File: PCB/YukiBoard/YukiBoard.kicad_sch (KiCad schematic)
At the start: 61 parts, among them J1 Conn_01x02, J2 Conn_01x02, SW1 SW_Push_45deg, SW10 SW_Push_45deg, SW11 SW_Push_45deg, SW12 SW_Push_45deg, SW13 SW_Push_45deg, SW14 SW_Push_45deg, SW15 SW_Push_45deg, SW16 SW_Push_45deg, SW17 SW_Push_45deg, SW18 SW_Push_45deg, SW19 SW_Push_45deg, SW2 SW_Push_45deg, SW20 SW_Push_45deg, SW21 SW_Push_45deg, SW22 SW_Push_45deg, SW23 SW_Push_45deg, SW24 SW_Push_45deg, SW25 SW_Push_45deg, SW26 SW_Push_45deg, SW27 SW_Push_45deg, SW28 SW_Push_45deg, SW29 SW_Push_45deg, SW3 SW_Push_45deg, SW30 SW_Push_45deg, SW31 SW_Push_45deg, SW32 SW_Push_45deg, SW33 SW_Push_45deg, SW34 SW_Push_45deg, SW35 SW_Push_45deg, SW36 SW_Push_45deg, SW37 SW_Push_45deg, SW38 SW_Push_45deg, SW39 SW_SPDT, SW4 SW_Push_45deg, SW5 SW_Push_45deg, SW6 SW_Push_45deg, SW7 SW_Push_45deg, SW8 SW_Push_45deg, SW9 SW_Push_45deg, U1 XIAO-nRF52840-DIP

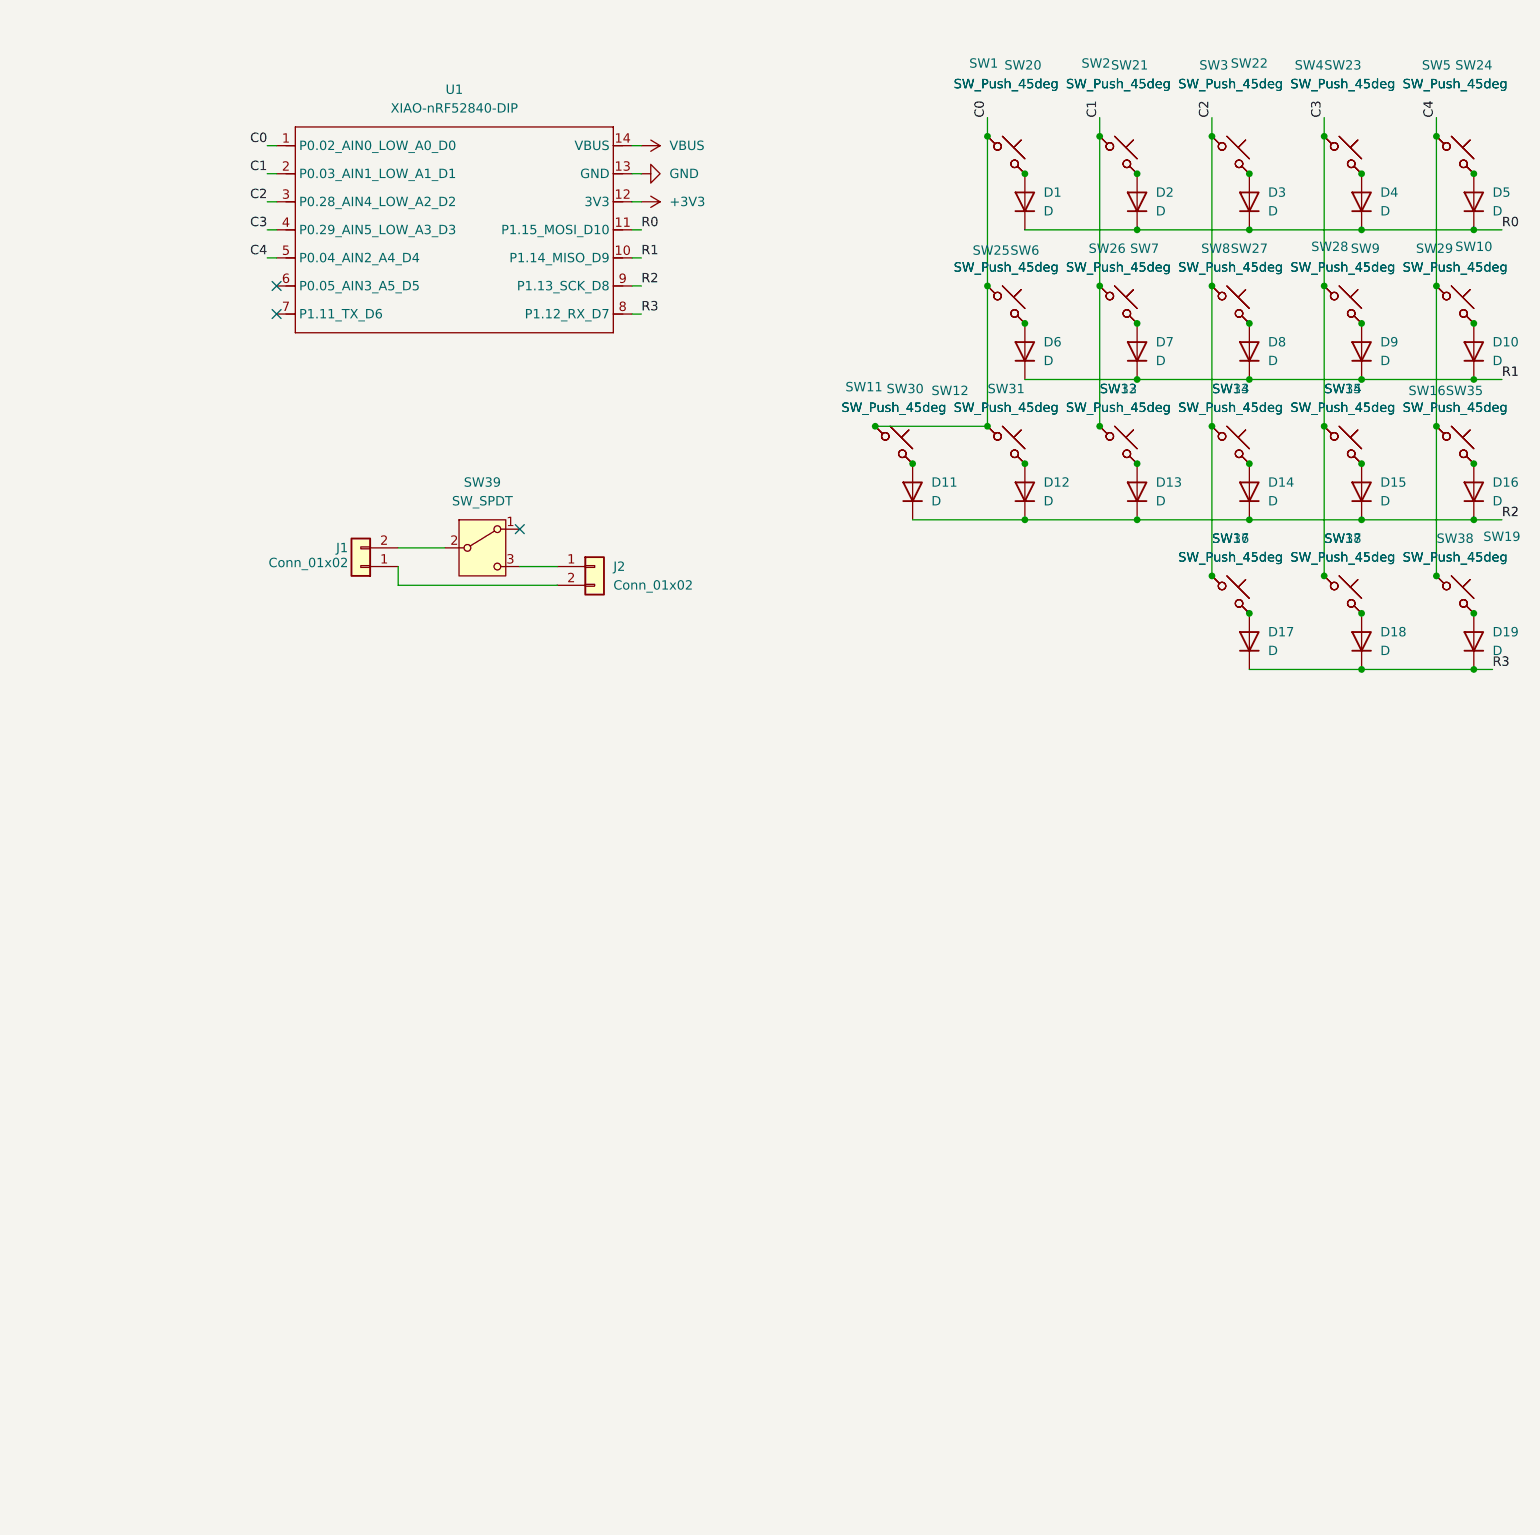
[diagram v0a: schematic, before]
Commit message: Add cool stuff to pcb 󰇳
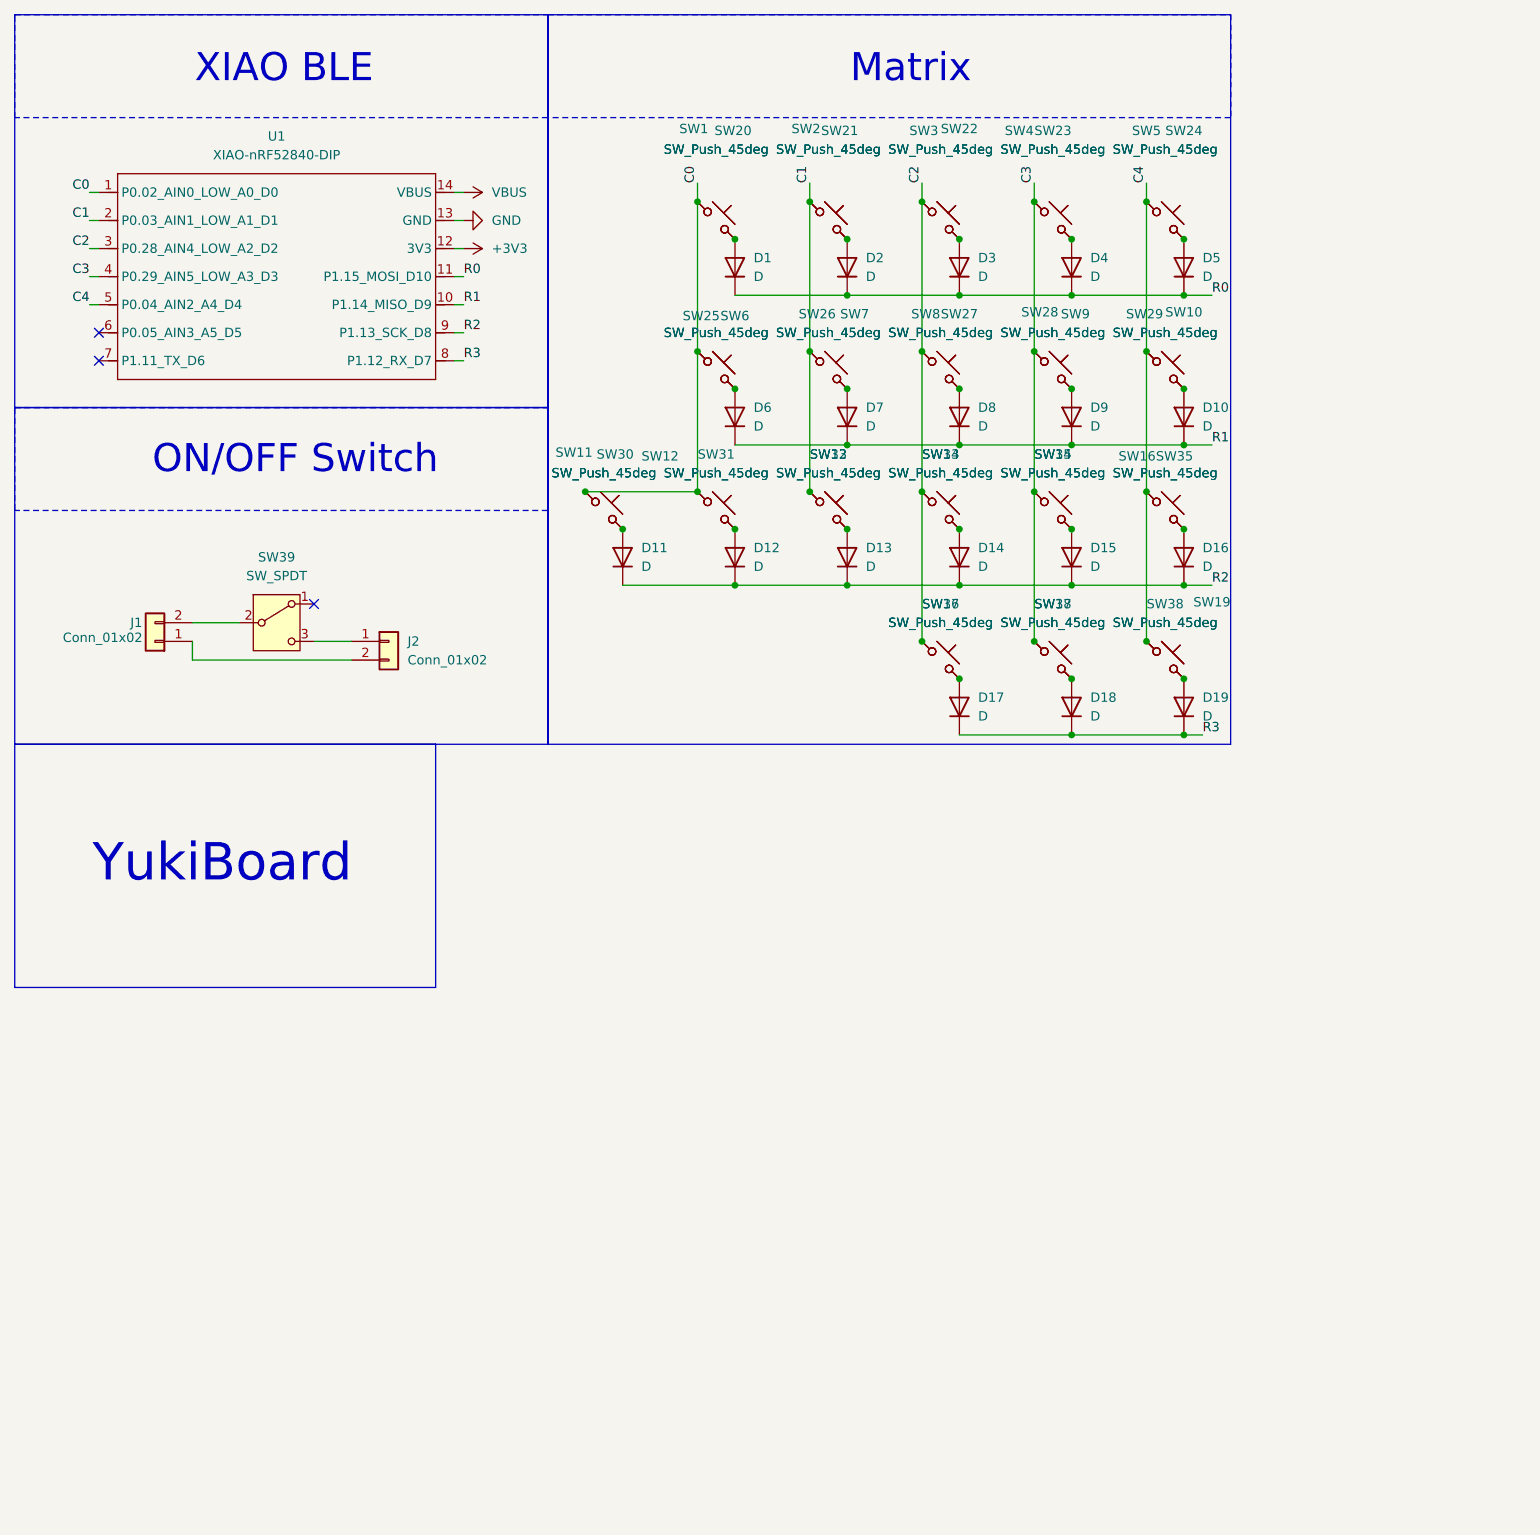
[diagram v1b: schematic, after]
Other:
- note added: "Matrix"
- note added: "ON/OFF Switch"
- note added: "XIAO BLE"
- note added: "YukiBoard"
- company: (none) -> manni
- title: (none) -> YukiBoard
- moved on the sheet: D1, D10, D11, D12, D13, D14, D15, D16, D17, D18, D19, D2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

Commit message: Add stuf
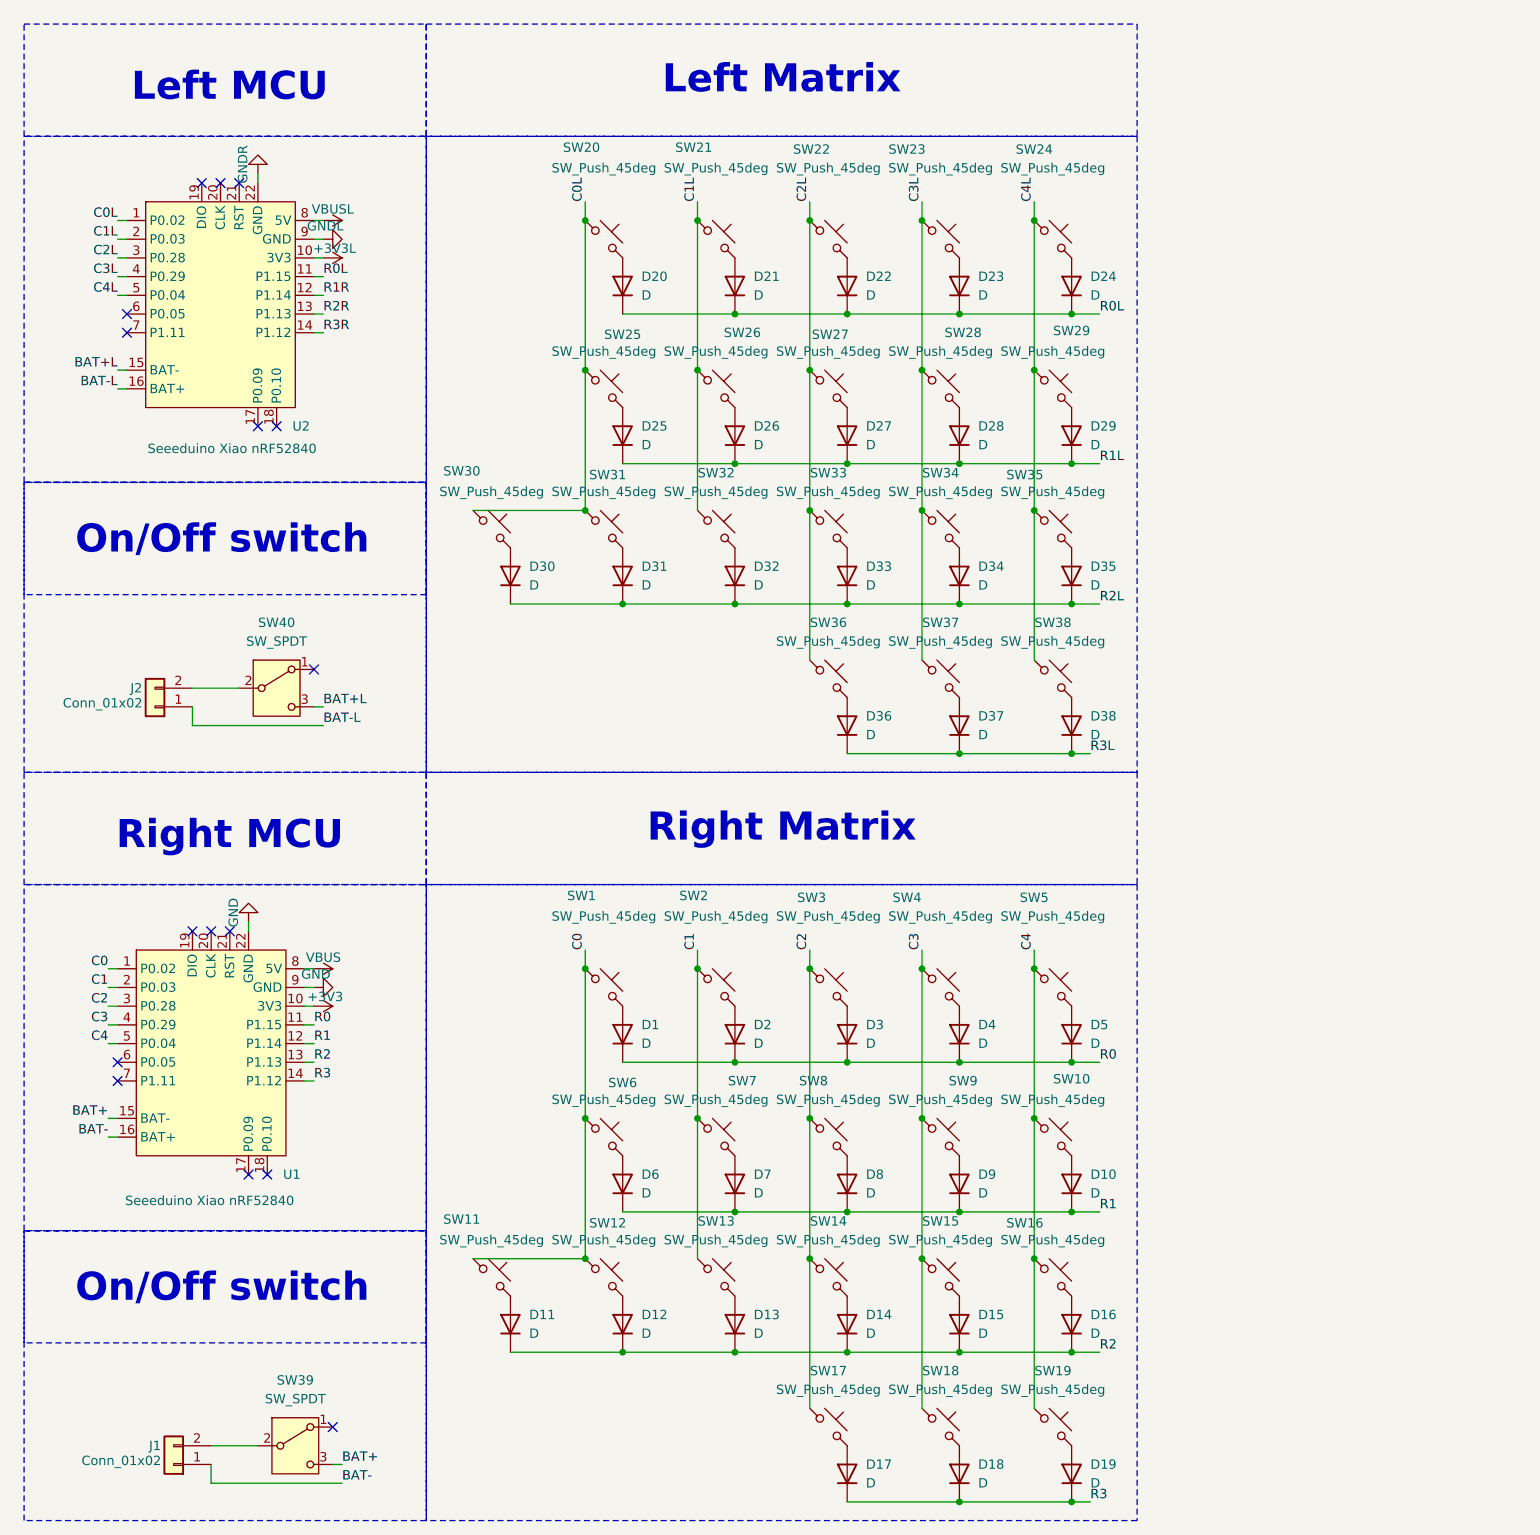
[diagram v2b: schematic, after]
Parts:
- removed U1: XIAO-nRF52840-DIP, XIAO-:XIAO-nRF52840-DIP, symbol Seeed_Studio_XIAO_Series:XIAO-nRF52840-DIP
- added D20, D21, D22, D23, D24, D25, D26, D27, D28, D29, D30, D31, D32, D33, D34, D35, D36, D37, D38: D, Diode_SMD:D_SOD-123, symbol Device:D
- added SW40: SW_SPDT, ScottoKeebs_Components:Switch_MSK12C02, symbol Switch:SW_SPDT
- added U1, U2: Seeeduino Xiao nRF52840, PCM_marbastlib-xp-promicroish:Xiao_nRF52840_ACH, symbol PCM_marbastlib-promicroish:Seeeduino_Xiao_nRF52840
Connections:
- net +3V3: now also U1.10 (3V3)
- net C0: now also U1.1 (P0.02); no longer SW20.1, SW25.1, SW30.1, SW31.1
- net C1: now also U1.2 (P0.03); no longer SW21.1, SW26.1, SW32.1
- net C2: now also U1.3 (P0.28); no longer SW22.1, SW27.1, SW33.1, SW36.1
- net C3: now also U1.4 (P0.29); no longer SW23.1, SW28.1, SW34.1, SW37.1
- net C4: now also U1.5 (P0.04); no longer SW24.1, SW29.1, SW35.1, SW38.1
- net GND: now also U1.22 (GND), U1.9 (GND)
- net R0: now also U1.11 (P1.15)
- net R1: now also U1.12 (P1.14)
- net R2: now also U1.13 (P1.13)
- net R3: now also U1.14 (P1.12)
- net VBUS: now also U1.8 (5V)
- net at D17.2 (A), SW17.2: no longer SW36.2
- net at D6.2 (A), SW6.2: no longer SW25.2
- net at D11.2 (A), SW11.2: no longer SW30.2
- net at D8.2 (A), SW8.2: no longer SW27.2
- net at D18.2 (A), SW18.2: no longer SW37.2
- net at D10.2 (A), SW10.2: no longer SW29.2
- net at D13.2 (A), SW13.2: no longer SW32.2
- net at D7.2 (A), SW7.2: no longer SW26.2
- net at D2.2 (A), SW2.2: no longer SW21.2
- net at D16.2 (A), SW16.2: no longer SW35.2
- net BAT+: now reaches SW39.3 (C)
- net BAT+: now also U1.15 (BAT-); no longer J2.1 (Pin_1)
- net at D4.2 (A), SW4.2: no longer SW23.2
- net at D19.2 (A), SW19.2: no longer SW38.2
- net at D1.2 (A), SW1.2: no longer SW20.2
- net at D3.2 (A), SW3.2: no longer SW22.2
- net at D15.2 (A), SW15.2: no longer SW34.2
- net at D12.2 (A), SW12.2: no longer SW31.2
- net at D14.2 (A), SW14.2: no longer SW33.2
- net at D9.2 (A), SW9.2: no longer SW28.2
- net at D5.2 (A), SW5.2: no longer SW24.2
- net at J2.2 (Pin_2): now also SW40.2 (B); no longer J1.1 (Pin_1)
- new net: D29.2 (A), SW29.2
- new net: D22.2 (A), SW22.2
- new net: D28.2 (A), SW28.2
- new net: D20.2 (A), SW20.2
- new net: D36.2 (A), SW36.2
- new net: D34.2 (A), SW34.2
- new net: D21.2 (A), SW21.2
- new net: D23.2 (A), SW23.2
- new net: D24.2 (A), SW24.2
- new net: D27.2 (A), SW27.2
- new net: D33.2 (A), SW33.2
- new net: D38.2 (A), SW38.2
- new net: D37.2 (A), SW37.2
- new net: D26.2 (A), SW26.2
- new net: D31.2 (A), SW31.2
- new net: D32.2 (A), SW32.2
- new net: D35.2 (A), SW35.2
- new net: D30.2 (A), SW30.2
- new net: D25.2 (A), SW25.2
- new net +3V3L: U2.10 (3V3)
- new net BAT+L: SW40.3 (C), U2.15 (BAT-)
- new net BAT-: J1.1 (Pin_1), U1.16 (BAT+)
- new net BAT-L: J2.1 (Pin_1), U2.16 (BAT+)
- new net C0L: SW20.1, SW25.1, SW30.1, SW31.1, U2.1 (P0.02)
- new net C1L: SW21.1, SW26.1, SW32.1, U2.2 (P0.03)
- new net C2L: SW22.1, SW27.1, SW33.1, SW36.1, U2.3 (P0.28)
- new net C3L: SW23.1, SW28.1, SW34.1, SW37.1, U2.4 (P0.29)
- new net C4L: SW24.1, SW29.1, SW35.1, SW38.1, U2.5 (P0.04)
- new net GNDL: U2.9 (GND)
- new net GNDR: U2.22 (GND)
- new net R0L: D20.1 (K), D21.1 (K), D22.1 (K), D23.1 (K), D24.1 (K), U2.11 (P1.15)
- new net R1L: D25.1 (K), D26.1 (K), D27.1 (K), D28.1 (K), D29.1 (K)
- new net R1R: U2.12 (P1.14)
- new net R2L: D30.1 (K), D31.1 (K), D32.1 (K), D33.1 (K), D34.1 (K), D35.1 (K)
- new net R2R: U2.13 (P1.13)
- new net R3L: D36.1 (K), D37.1 (K), D38.1 (K)
- new net R3R: U2.14 (P1.12)
- new net VBUSL: U2.8 (5V)
- no-connect marks 3 -> 16
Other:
- note added: "Left MCU"
- note added: "Left Matrix"
- note added: "On/Off switch"
- note added: "Right MCU"
- note added: "Right Matrix"
- note removed: "Matrix"
- note removed: "ON/OFF Switch"
- note removed: "XIAO BLE"
- note removed: "YukiBoard"
- moved on the sheet: D1, D10, D11, D12, D13, D14, D15, D16, D17, D18, D19, D2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
